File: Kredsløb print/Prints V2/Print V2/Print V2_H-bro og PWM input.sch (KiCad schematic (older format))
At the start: 19 parts, among them J19 Conn_01x01_Male, J20 Conn_01x01_Male, J27 Conn_01x01_Male, J28 Conn_01x01_Male, J29 Conn_01x01_Male, J30 Conn_01x01_Male, J31 Conn_01x01_Male, J32 Conn_01x01_Male, Q17 BC547, Q20 BC547, Q21 TIP127, Q22 TIP120, Q24 TIP120, Q27 TIP127, Q28 TIP120, U3 4049

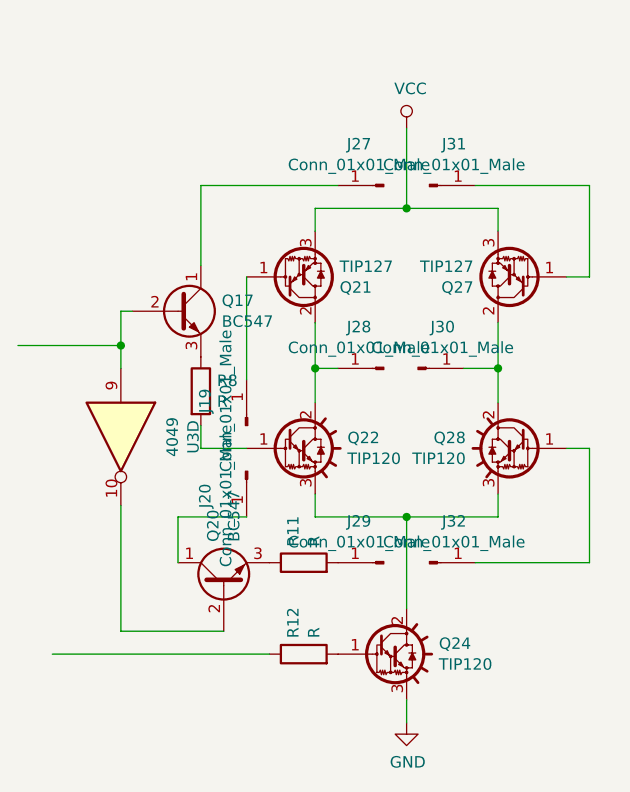
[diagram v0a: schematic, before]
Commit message: Lotsa stuff
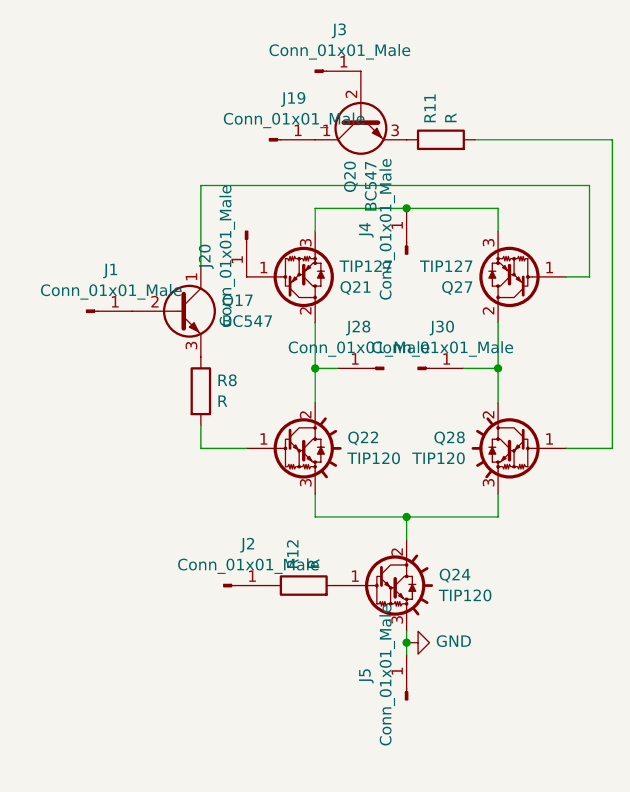
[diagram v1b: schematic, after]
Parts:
- removed J27, J29, J31, J32: Conn_01x01_Male, Connector_PinHeader_1.00mm:PinHeader_1x01_P1.00mm_Vertical, symbol Connector:Conn_01x01_Male
- removed U3: 4049, Package_DIP:DIP-16_W7.62mm_LongPads, symbol 4xxx:4049
- added J1, J2, J3, J4, J5: Conn_01x01_Male, Connector_PinHeader_2.54mm:PinHeader_1x01_P2.54mm_Vertical, symbol Connector:Conn_01x01_Male
- J19, J20, J28, J30: footprint Connector_PinHeader_1.00mm:PinHeader_1x01_P1.00mm_Vertical -> Connector_PinHeader_2.54mm:PinHeader_1x01_P2.54mm_Vertical
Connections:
- net labels removed: VCC
- wire segments 37 -> 26
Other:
- moved on the sheet: J19, J20, Q20, Q24, R11, R12
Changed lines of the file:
@@
 EESchema Schematic File Version 4
+LIBS:Print V2_H-bro og PWM input-cache
 EELAYER 29 0
 EELAYER END
@@
 L Print-V2-rescue:TIP120-00-OTG-Transistor Q24
 U 1 1 5CB310D8
-P 5500 4600
-F 0 "Q24" H 5741 4646 50  0000 L CNN
-F 1 "TIP120" H 5741 4555 50  0000 L CNN
-F 2 "Package_TO_SOT_THT:TO-220-3_Vertical" H 5750 4525 50  0001 L CIN
-F 3 "http://www.fairchildsemi.com/ds/TI/TIP120.pdf" H 5500 4600 50  0001 L CNN
-	1    5500 4600
+P 5500 4300
+F 0 "Q24" H 5741 4346 50  0000 L CNN
+F 1 "TIP120" H 5741 4255 50  0000 L CNN
+F 2 "Package_TO_SOT_THT:TO-220-3_Vertical" H 5750 4225 50  0001 L CIN
+F 3 "http://www.fairchildsemi.com/ds/TI/TIP120.pdf" H 5500 4300 50  0001 L CNN
+	1    5500 4300
 	1    0    0    -1
 $EndComp
@@
 F 0 "J30" H 5758 3531 50  0000 C CNN
 F 1 "Conn_01x01_Male" H 5758 3440 50  0000 C CNN
-F 2 "Connector_PinHeader_1.00mm:PinHeader_1x01_P1.00mm_Vertical" H 5650 3350 50  0001 C CNN
+F 2 "Connector_PinHeader_2.54mm:PinHeader_1x01_P2.54mm_Vertical" H 5650 3350 50  0001 C CNN
 F 3 "~" H 5650 3350 50  0001 C CNN
 	1    5650 3350
@@
 F 0 "J28" H 5608 3531 50  0000 C CNN
 F 1 "Conn_01x01_Male" H 5608 3440 50  0000 C CNN
-F 2 "Connector_PinHeader_1.00mm:PinHeader_1x01_P1.00mm_Vertical" H 5500 3350 50  0001 C CNN
+F 2 "Connector_PinHeader_2.54mm:PinHeader_1x01_P2.54mm_Vertical" H 5500 3350 50  0001 C CNN
 F 3 "~" H 5500 3350 50  0001 C CNN
 	1    5500 3350
@@
 Wire Wire Line
 	5200 4000 5200 3900
-Wire Wire Line
-	5600 4400 5600 4000
 Connection ~ 5600 4000
 Wire Wire Line
@@
 Wire Wire Line
 	6000 2650 6000 2750
-$Comp
-L power:GND #PWR0104
-U 1 1 5CB310FD
-P 5600 4900
-F 0 "#PWR0104" H 5600 4650 50  0001 C CNN
-F 1 "GND" H 5605 4727 50  0000 C CNN
-F 2 "" H 5600 4900 50  0001 C CNN
-F 3 "" H 5600 4900 50  0001 C CNN
-	1    5600 4900
-	1    0    0    -1
-$EndComp
 $Comp
 L Print-V2-rescue:BC547-00-OTG-Transistor Q20
 U 1 1 5CB31103
-P 4800 4300
-F 0 "Q20" H 4991 4346 50  0000 L CNN
-F 1 "BC547" H 4991 4255 50  0000 L CNN
-F 2 "Package_TO_SOT_THT:TO-92_Inline" H 5000 4225 50  0001 L CIN
-F 3 "http://www.fairchildsemi.com/ds/BC/BC547.pdf" H 4800 4300 50  0001 L CNN
-	1    4800 4300
-	0    -1   -1   0
+P 5400 2250
+F 0 "Q20" H 5591 2296 50  0000 L CNN
+F 1 "BC547" H 5591 2205 50  0000 L CNN
+F 2 "Package_TO_SOT_THT:TO-92_Inline" H 5600 2175 50  0001 L CIN
+F 3 "http://www.fairchildsemi.com/ds/BC/BC547.pdf" H 5400 2250 50  0001 L CNN
+	1    5400 2250
+	0    -1   1    0
 $EndComp
 $Comp
 L Device:R R11
 U 1 1 5CB31109
-P 5150 4200
-F 0 "R11" H 5220 4246 50  0000 L CNN
-F 1 "R" H 5220 4155 50  0000 L CNN
-F 2 "footprints otg:R_vandret" V 5080 4200 50  0001 C CNN
-F 3 "~" H 5150 4200 50  0001 C CNN
-	1    5150 4200
-	0    -1   -1   0
-$EndComp
-$Comp
-L Connector:Conn_01x01_Male J29
-U 1 1 5CB3110F
-P 5500 4200
-F 0 "J29" H 5608 4381 50  0000 C CNN
-F 1 "Conn_01x01_Male" H 5608 4290 50  0000 C CNN
-F 2 "Connector_PinHeader_1.00mm:PinHeader_1x01_P1.00mm_Vertical" H 5500 4200 50  0001 C CNN
-F 3 "~" H 5500 4200 50  0001 C CNN
-	1    5500 4200
-	-1   0    0    -1
-$EndComp
-$Comp
-L Connector:Conn_01x01_Male J32
-U 1 1 5CB31115
-P 5700 4200
-F 0 "J32" H 5808 4381 50  0000 C CNN
-F 1 "Conn_01x01_Male" H 5808 4290 50  0000 C CNN
-F 2 "Connector_PinHeader_1.00mm:PinHeader_1x01_P1.00mm_Vertical" H 5700 4200 50  0001 C CNN
-F 3 "~" H 5700 4200 50  0001 C CNN
-	1    5700 4200
-	1    0    0    -1
+P 5750 2350
+F 0 "R11" H 5820 2396 50  0000 L CNN
+F 1 "R" H 5820 2305 50  0000 L CNN
+F 2 "footprints otg:R_vandret" V 5680 2350 50  0001 C CNN
+F 3 "~" H 5750 2350 50  0001 C CNN
+	1    5750 2350
+	0    -1   -1   0
 $EndComp
 $Comp
@@
 Wire Wire Line
 	4700 3700 4700 3600
-Wire Wire Line
-	5900 4200 6400 4200
-Wire Wire Line
-	6400 4200 6400 3700
-Wire Wire Line
-	6400 3700 6300 3700
 $Comp
 L Connector:Conn_01x01_Male J20
 U 1 1 5CB3112E
-P 4900 3800
-F 0 "J20" H 5008 3981 50  0000 C CNN
-F 1 "Conn_01x01_Male" H 5008 3890 50  0000 C CNN
-F 2 "Connector_PinHeader_1.00mm:PinHeader_1x01_P1.00mm_Vertical" H 4900 3800 50  0001 C CNN
-F 3 "~" H 4900 3800 50  0001 C CNN
-	1    4900 3800
+P 4900 2750
+F 0 "J20" H 5008 2931 50  0000 C CNN
+F 1 "Conn_01x01_Male" H 5008 2840 50  0000 C CNN
+F 2 "Connector_PinHeader_2.54mm:PinHeader_1x01_P2.54mm_Vertical" H 4900 2750 50  0001 C CNN
+F 3 "~" H 4900 2750 50  0001 C CNN
+	1    4900 2750
 	0    -1   1    0
 $EndComp
@@
 L Connector:Conn_01x01_Male J19
 U 1 1 5CB31134
-P 4900 3600
-F 0 "J19" H 5008 3781 50  0000 C CNN
-F 1 "Conn_01x01_Male" H 5008 3690 50  0000 C CNN
-F 2 "Connector_PinHeader_1.00mm:PinHeader_1x01_P1.00mm_Vertical" H 4900 3600 50  0001 C CNN
-F 3 "~" H 4900 3600 50  0001 C CNN
-	1    4900 3600
-	0    -1   -1   0
+P 5000 2350
+F 0 "J19" H 5108 2531 50  0000 C CNN
+F 1 "Conn_01x01_Male" H 5108 2440 50  0000 C CNN
+F 2 "Connector_PinHeader_2.54mm:PinHeader_1x01_P2.54mm_Vertical" H 5000 2350 50  0001 C CNN
+F 3 "~" H 5000 2350 50  0001 C CNN
+	1    5000 2350
+	1    0    0    -1
 $EndComp
 Wire Wire Line
@@
 L Device:R R12
 U 1 1 5CB3113B
-P 5150 4600
-F 0 "R12" H 5220 4646 50  0000 L CNN
-F 1 "R" H 5220 4555 50  0000 L CNN
-F 2 "footprints otg:R_vandret" V 5080 4600 50  0001 C CNN
-F 3 "~" H 5150 4600 50  0001 C CNN
-	1    5150 4600
+P 5150 4300
+F 0 "R12" H 5220 4346 50  0000 L CNN
+F 1 "R" H 5220 4255 50  0000 L CNN
+F 2 "footprints otg:R_vandret" V 5080 4300 50  0001 C CNN
+F 3 "~" H 5150 4300 50  0001 C CNN
+	1    5150 4300
 	0    -1   -1   0
 $EndComp
@@
 $EndComp
 Wire Wire Line
-	4600 4200 4600 4000
-Wire Wire Line
-	4600 4000 4900 4000
-Wire Wire Line
-	4800 4500 4350 4500
-Wire Wire Line
-	4350 4500 4350 3950
-Wire Wire Line
-	4400 3100 4350 3100
-Wire Wire Line
-	5600 4900 5600 4800
-Wire Wire Line
-	4350 3100 4350 3250
-$Comp
-L power:VCC #PWR0105
-U 1 1 5CB3114E
-P 5600 2300
-F 0 "#PWR0105" H 5600 2150 50  0001 C CNN
-F 1 "VCC" H 5617 2473 50  0000 C CNN
-F 2 "" H 5600 2300 50  0001 C CNN
-F 3 "" H 5600 2300 50  0001 C CNN
-	1    5600 2300
-	1    0    0    -1
-$EndComp
+	5600 4600 5600 4550
 Wire Wire Line
 	5200 2650 5600 2650
-$Comp
-L Connector:Conn_01x01_Male J31
-U 1 1 5CB31155
-P 5700 2550
-F 0 "J31" H 5808 2731 50  0000 C CNN
-F 1 "Conn_01x01_Male" H 5808 2640 50  0000 C CNN
-F 2 "Connector_PinHeader_1.00mm:PinHeader_1x01_P1.00mm_Vertical" H 5700 2550 50  0001 C CNN
-F 3 "~" H 5700 2550 50  0001 C CNN
-	1    5700 2550
-	1    0    0    -1
-$EndComp
-$Comp
-L Connector:Conn_01x01_Male J27
-U 1 1 5CB3115B
-P 5500 2550
-F 0 "J27" H 5608 2731 50  0000 C CNN
-F 1 "Conn_01x01_Male" H 5608 2640 50  0000 C CNN
-F 2 "Connector_PinHeader_1.00mm:PinHeader_1x01_P1.00mm_Vertical" H 5500 2550 50  0001 C CNN
-F 3 "~" H 5500 2550 50  0001 C CNN
-	1    5500 2550
-	-1   0    0    -1
-$EndComp
 Wire Wire Line
 	6400 2950 6300 2950
@@
 	-1   0    0    1
 $EndComp
-Wire Wire Line
-	4900 3400 4900 2950
-Wire Wire Line
-	5300 2550 4700 2550
-Wire Wire Line
-	6400 2550 5900 2550
-Wire Wire Line
-	5600 2300 5600 2650
 Connection ~ 5600 2650
 Wire Wire Line
 	5600 2650 6000 2650
 $Comp
-L 4xxx:4049 U3
-U 4 1 5CB310F7
-P 4350 3650
-F 0 "U3" H 4350 3967 50  0000 C CNN
-F 1 "4049" H 4350 3876 50  0000 C CNN
-F 2 "Package_DIP:DIP-16_W7.62mm_LongPads" H 4350 3650 50  0001 C CNN
-F 3 "http://www.intersil.com/content/dam/intersil/documents/cd40/cd4049ubms.pdf" H 4350 3650 50  0001 C CNN
-	4    4350 3650
-	0    1    1    0
-$EndComp
-Wire Wire Line
-	3900 3250 4350 3250
-Connection ~ 4350 3250
-Wire Wire Line
-	4350 3250 4350 3350
-Wire Wire Line
-	5000 4600 4050 4600
+L Connector:Conn_01x01_Male J4
+U 1 1 5CAE1552
+P 5600 2850
+F 0 "J4" H 5708 3031 50  0000 C CNN
+F 1 "Conn_01x01_Male" H 5708 2940 50  0000 C CNN
+F 2 "Connector_PinHeader_2.54mm:PinHeader_1x01_P2.54mm_Vertical" H 5600 2850 50  0001 C CNN
+F 3 "~" H 5600 2850 50  0001 C CNN
+	1    5600 2850
+	0    -1   -1   0
+$EndComp
+Wire Wire Line
+	4700 2550 6400 2550
+Wire Wire Line
+	6500 3700 6500 2350
+Wire Wire Line
+	6500 2350 5900 2350
+Wire Wire Line
+	6300 3700 6500 3700
+Wire Wire Line
+	5600 4100 5600 4000
+$Comp
+L Connector:Conn_01x01_Male J1
+U 1 1 5CAEBDCC
+P 4200 3100
+F 0 "J1" H 4308 3281 50  0000 C CNN
+F 1 "Conn_01x01_Male" H 4308 3190 50  0000 C CNN
+F 2 "Connector_PinHeader_2.54mm:PinHeader_1x01_P2.54mm_Vertical" H 4200 3100 50  0001 C CNN
+F 3 "~" H 4200 3100 50  0001 C CNN
+	1    4200 3100
+	1    0    0    -1
+$EndComp
+$Comp
+L Connector:Conn_01x01_Male J3
+U 1 1 5CAEC4E3
+P 5200 2050
+F 0 "J3" H 5308 2231 50  0000 C CNN
+F 1 "Conn_01x01_Male" H 5308 2140 50  0000 C CNN
+F 2 "Connector_PinHeader_2.54mm:PinHeader_1x01_P2.54mm_Vertical" H 5200 2050 50  0001 C CNN
+F 3 "~" H 5200 2050 50  0001 C CNN
+	1    5200 2050
+	1    0    0    -1
+$EndComp
+$Comp
+L Connector:Conn_01x01_Male J2
+U 1 1 5CAECC3B
+P 4800 4300
+F 0 "J2" H 4908 4481 50  0000 C CNN
+F 1 "Conn_01x01_Male" H 4908 4390 50  0000 C CNN
+F 2 "Connector_PinHeader_2.54mm:PinHeader_1x01_P2.54mm_Vertical" H 4800 4300 50  0001 C CNN
+F 3 "~" H 4800 4300 50  0001 C CNN
+	1    4800 4300
+	1    0    0    -1
+$EndComp
+$Comp
+L Connector:Conn_01x01_Male J5
+U 1 1 5CAED36D
+P 5600 4800
+F 0 "J5" H 5708 4981 50  0000 C CNN
+F 1 "Conn_01x01_Male" H 5708 4890 50  0000 C CNN
+F 2 "Connector_PinHeader_2.54mm:PinHeader_1x01_P2.54mm_Vertical" H 5600 4800 50  0001 C CNN
+F 3 "~" H 5600 4800 50  0001 C CNN
+	1    5600 4800
+	0    -1   -1   0
+$EndComp
+$Comp
+L power:GND #PWR0101
+U 1 1 5CB1B826
+P 5600 4550
+F 0 "#PWR0101" H 5600 4300 50  0001 C CNN
+F 1 "GND" V 5605 4422 50  0000 R CNN
+F 2 "" H 5600 4550 50  0001 C CNN
+F 3 "" H 5600 4550 50  0001 C CNN
+	1    5600 4550
+	0    -1   -1   0
+$EndComp
+Connection ~ 5600 4550
+Wire Wire Line
+	5600 4550 5600 4500
 $EndSCHEMATC
